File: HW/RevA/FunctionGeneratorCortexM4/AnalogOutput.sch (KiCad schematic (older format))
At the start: 37 parts, among them U11 LTC6910, U12 TL072, U13 TL072, U4 SN74LVC1G3157DCKR

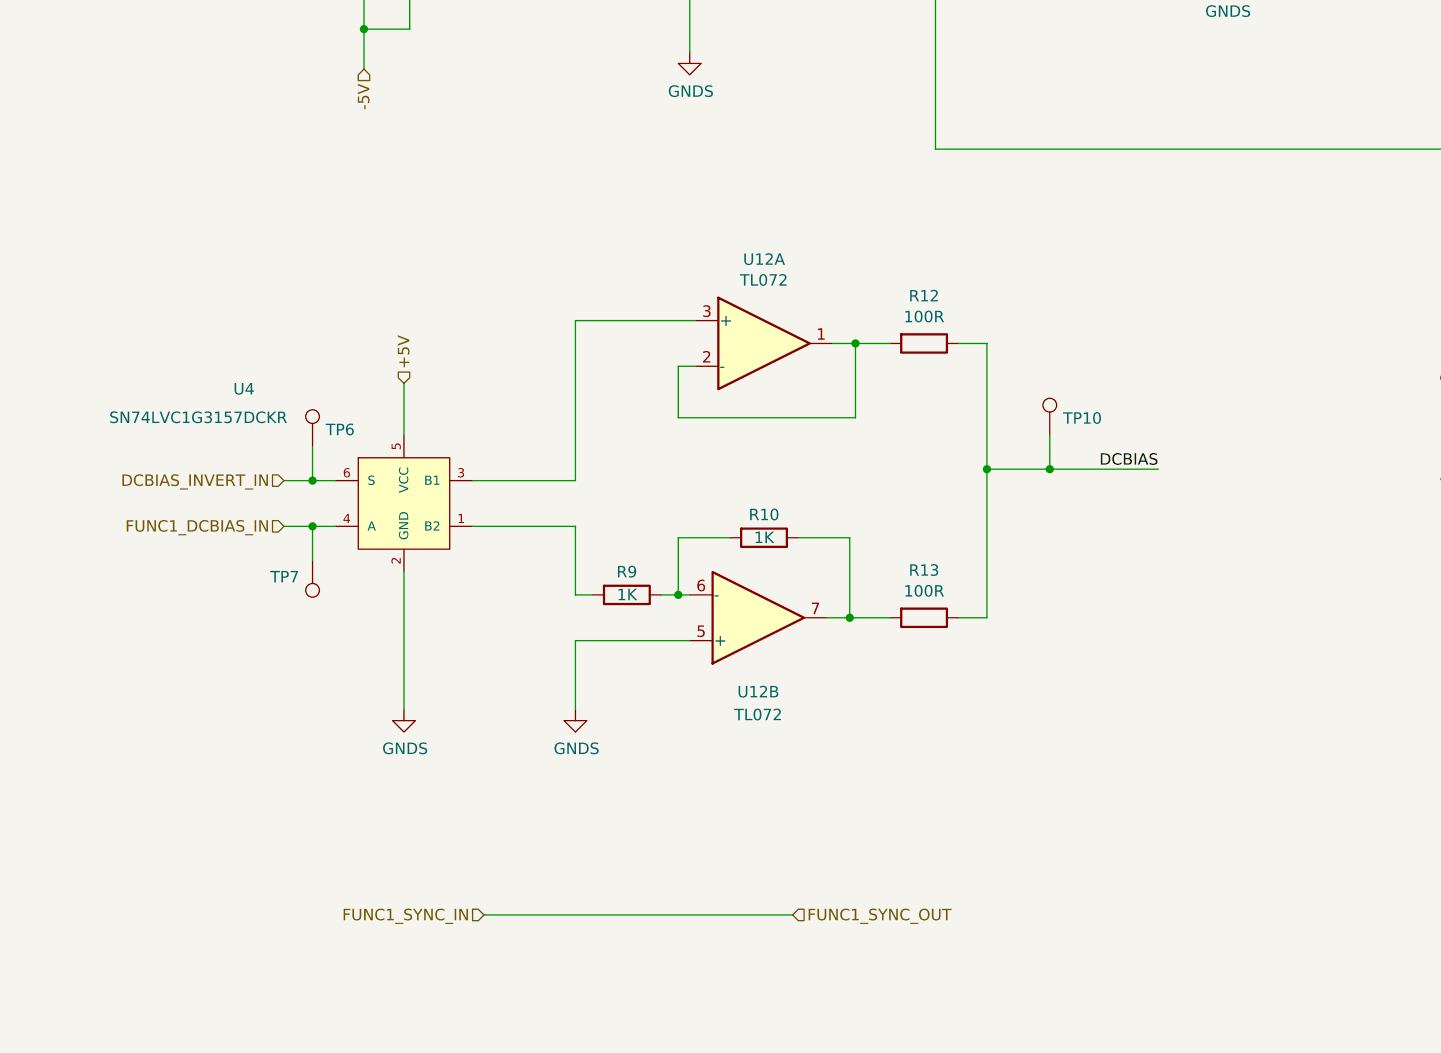
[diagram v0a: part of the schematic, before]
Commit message: updated RevA
Generated GERBERS
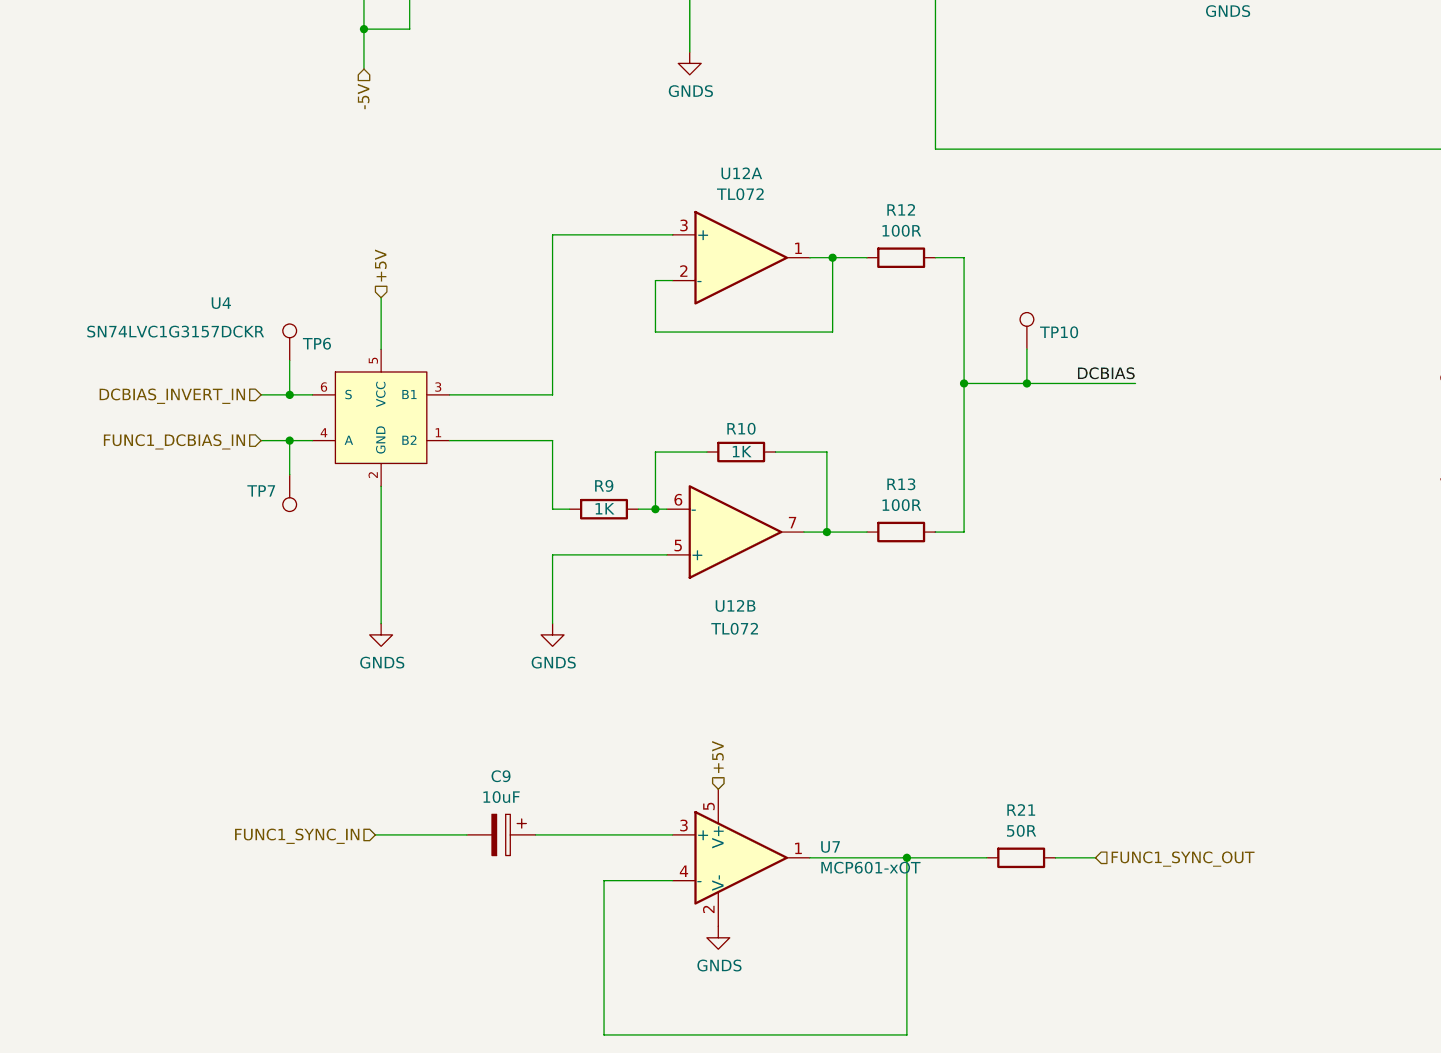
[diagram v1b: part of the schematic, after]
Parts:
- added C9: 10uF, Capacitor_SMD:CP_Elec_4x5.7, symbol Device:CP
- added R21: 50R, Resistor_SMD:R_1206_3216Metric_Pad1.42x1.75mm_HandSolder, symbol Device:R
- added U7: MCP601-xOT, Package_TO_SOT_SMD:SOT-23-5, symbol Amplifier_Operational:MCP601-xOT
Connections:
- net +5V: now also U7.5 (V+)
- net FUNC1_SYNC_IN: now also C9.2
- net GNDS: now also U7.2 (V-)
- new net: R21.2, U7.1, U7.4 (-)
- new net: C9.1, U7.3 (+)
- new net FUNC1_SYNC_OUT: R21.1
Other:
- moved on the sheet: R10, R12, R13, R9, TP10, TP6, TP7, U12A, U12B, U4
